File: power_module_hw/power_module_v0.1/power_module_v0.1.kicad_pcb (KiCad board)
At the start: 2 copper layers, 35 x 23 mm, 48 parts, among them Q1 BSS138, U3 INA226, U4 LDK130-ADJ_DFN6

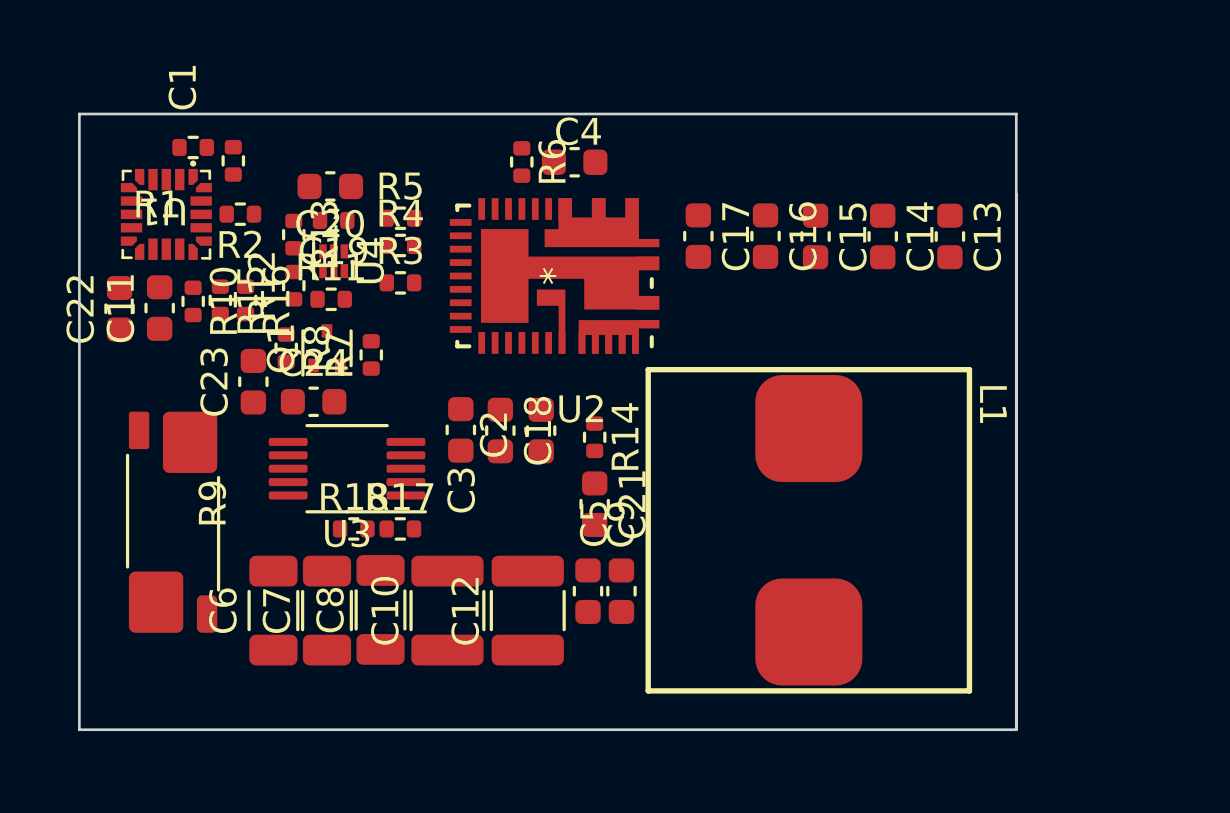
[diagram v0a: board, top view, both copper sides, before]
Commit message: update the design
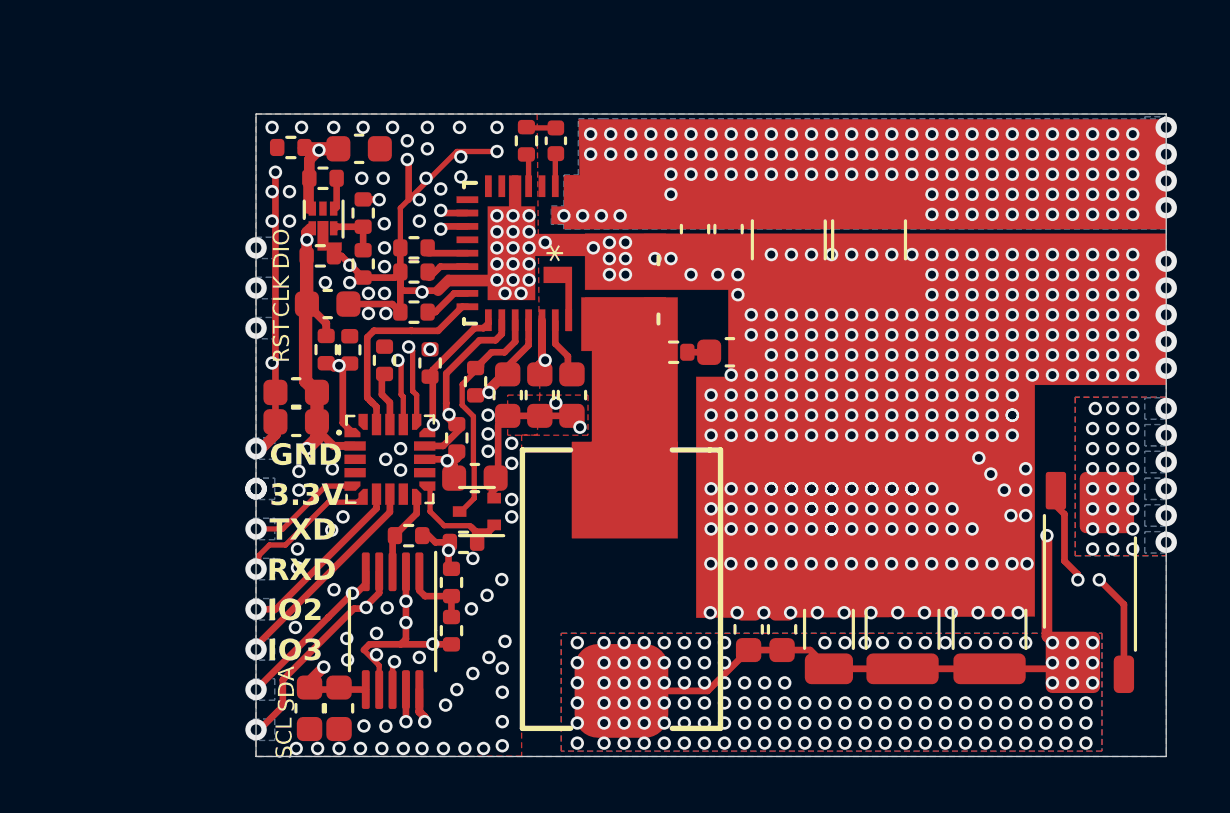
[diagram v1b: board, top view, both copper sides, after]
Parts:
- C10, C12, C9: value 0.1uF -> 47uF
- C11, C20: value 0.1uF -> 22uF
- C13, C14: value 0.1uF -> 47uF; footprint Capacitor_SMD:C_0603_1608Metric -> Capacitor_SMD:C_1210_3225Metric
- C15: value 0.1uF -> 10pF
- C2, C3: value 0.1uF -> 1uF
- C4: footprint Capacitor_SMD:C_0603_1608Metric -> Capacitor_SMD:C_0402_1005Metric
- C6: value 0.1uF -> 100pF
- C7: value 0.1uF -> 22uF; footprint Capacitor_SMD:C_1206_3216Metric -> Capacitor_SMD:C_0603_1608Metric
- C8: footprint Capacitor_SMD:C_1206_3216Metric -> Resistor_SMD:R_0402_1005Metric
- R1, R10, R11, R5, R7, R8: value 1M -> 10K
- R12: value 1M -> 31.2K 1%
- R13: value 1M -> 10K 1%
- R14: value 1M -> 1K
- R15, R16: value 1M -> 4.7K
- R17: value 1M -> NC
- R18, R2, R6: value 1M -> 0R
- R3: value 1M -> 2.87K
- R4: value 1M -> 2.32K
- R9: value R_Shunt_US -> 20mR
- U1: value ~ -> GD32E230F4V6TR
- U2: value ~ -> SiC45X
- moved R9 34.3 mm to (147.8, 107.5)
- moved C6 20.8 mm to (138.0, 109.2)
- moved C8 17.6 mm to (117.9, 91.2), turned to 180 degrees
- moved C7 17.3 mm to (120.5, 91.3), turned to 0 degrees
- moved C12 17.3 mm to (144.0, 109.2)
- moved C10 17.0 mm to (140.8, 109.2)
- moved U1 12.4 mm to (121.6, 102.9), turned to 0 degrees
- moved C23 12.4 mm to (118.6, 112.2), turned to -90 degrees
- moved C17 12.3 mm to (124.8, 103.6), turned to 0 degrees
- moved R10 11.9 mm to (122.3, 105.8), turned to 0 degrees
- moved C24 11.5 mm to (119.7, 112.2), turned to -90 degrees
- moved R8 9.82 mm to (124.3, 106.0), turned to 0 degrees
- moved R16 9.42 mm to (124.1, 102.1)
- moved R1 9.04 mm to (119.2, 98.8), turned to 90 degrees
- moved C1 8.29 mm to (120.1, 98.8), turned to -90 degrees
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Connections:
- net GPIO0 renamed SWDIO
- net GPIO1 renamed SWCLK
- C1 pad 1: GNDD -> GNDA
- C17 pad 1: VCC -> +3.3V
- C7 pad 1: Net-(U2-VSEN+) -> +5VA
- C8 pad 1: Net-(U2-VSEN+) -> +5VA
- R15 pad 1: I2IC0_SDA -> I2C0_SDA
- R18 pad 1: GNDD -> GNDA
- R2 pad 1: GNDD -> GNDA
- U1 pad 10: unconnected-(U1-PA7-Pad10) -> ~{SENSOR_ALERT}
- U1 pad 11: GPIO2 -> ~{PWR_EN}
- U1 pad 12: GNDD -> GNDA
- U1 pad 19: unconnected-(U1-OSCIN-Pad19) -> PWR_ALERT
- U1 pad 4: UART_TXD -> unconnected-(U1-PA1-Pad4)
- U1 pad 5: UART_RXD -> UART_TXD
- U1 pad 6: ~{SENSOR_ALERT} -> UART_RXD
- U1 pad 7: PWR_ALERT -> GPIO2
- U1 pad 8: ~{PWR_EN} -> GPIO3
- U3 pad 2: GNDD -> GNDA
- U3 pad 4: I2IC0_SDA -> I2C0_SDA
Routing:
- net GNDA: track 0.00 -> 121.1 mm, vias 0 -> 390
- net Net-(U2-VSEN+): track 0.00 -> 81.5 mm, vias 0 -> 128
- net +3.3V: track 0.00 -> 57.1 mm, vias 0 -> 9
- net Net-(U3-Vin+): track 0.00 -> 33.2 mm, vias 0 -> 2
- net Net-(U3-Vin-): track 0.00 -> 32.6 mm, vias 0 -> 2
- net I2C0_SCL: track 0.00 -> 23.1 mm, vias 0 -> 3
- net I2C0_SDA: track 0.00 -> 22.2 mm, vias 0 -> 3
- net +5VA: track 0.00 -> 21.3 mm, vias 0 -> 2
- net VCC: track 0.00 -> 15.7 mm, vias 0 -> 112
- net SWDIO: track 0.00 -> 10.5 mm, vias 0 -> 2
- net SWCLK: track 0.00 -> 8.80 mm, vias 0 -> 2
- net Net-(Q1-D): track 0.00 -> 8.46 mm
- net GPIO3: track 0.00 -> 7.82 mm, vias 0 -> 1
- net PWR_ALERT: track 0.00 -> 7.72 mm
- net Net-(U1-NRST): track 0.00 -> 6.50 mm, vias 0 -> 2
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- added copper zone on B.Cu, net +3.3V
- added copper zone on B.Cu, net /VOUT
- added copper zone on F.Cu, net /VOUT
- added copper zone on In1.Cu, net /VOUT
- added copper zone on In2.Cu, net /VOUT
- added copper zone on B.Cu, net GNDA
- added copper zone on F.Cu, net GNDA
- added copper zone on In1.Cu, net GNDA
- added copper zone on In2.Cu, net GNDA
- added copper zone on B.Cu, net GPIO2
- added copper zone on B.Cu, net GPIO3
- added copper zone on B.Cu, net I2C0_SCL
- added copper zone on B.Cu, net I2C0_SDA
- added copper zone on B.Cu, net Net-(U1-NRST)
- added copper zone on B.Cu, net Net-(U2-VSEN+)
- added copper zone on F.Cu, net Net-(U2-VSEN+)
- added copper zone on In1.Cu, net Net-(U2-VSEN+)
- added copper zone on In2.Cu, net Net-(U2-VSEN+)
- added copper zone on B.Cu, net SWCLK
- added copper zone on B.Cu, net SWDIO
- added copper zone on B.Cu, net UART_RXD
- added copper zone on B.Cu, net UART_TXD
- added copper zone on B.Cu, net VCC
- added copper zone on In1.Cu, net VCC
- added copper zone on In2.Cu, net VCC
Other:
- board size 35 x 23 mm -> 34 x 24 mm
- copper layers 2 -> 4
- board text added: "3.3V"
- board text added: "CLK"
- board text added: "DIO"
- board text added: "GND"
- board text added: "IO2"
- board text added: "IO3"
- board text added: "RST"
- board text added: "RXD"
- board text added: "SCL"
- board text added: "SDA"
- board text added: "TXD"
